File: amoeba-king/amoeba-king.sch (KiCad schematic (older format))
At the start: 6 parts, among them J1 Conn_01x05_Male, J2 Conn_01x05_Male, J3 Conn_01x04_Male, J4 Conn_01x05_Male, J5 Conn_01x01_Male, J6 Conn_01x01_Male

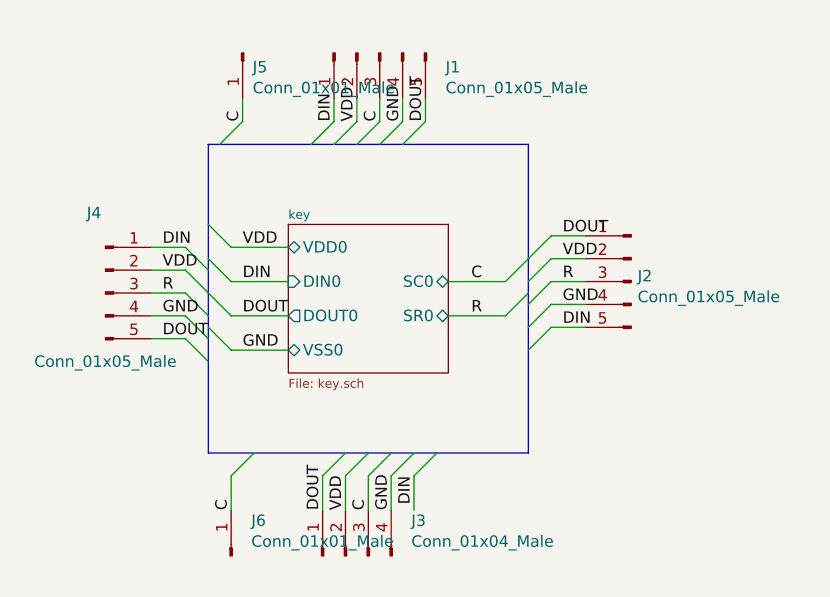
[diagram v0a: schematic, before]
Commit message: Getting pretty close to v1.1 improved Pads
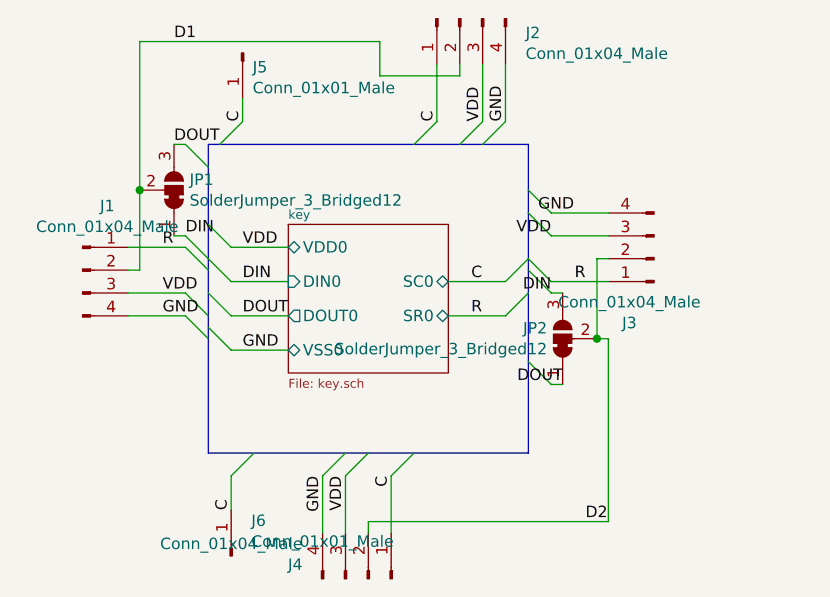
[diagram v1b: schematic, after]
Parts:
- removed J1, J2, J4: Conn_01x05_Male, amoeba-modules:Header_1x05_P1.27mm, symbol Connector:Conn_01x05_Male
- added J1, J4: Conn_01x04_Male, amoeba-modules:Header_1x04_P1.27mmL, symbol Connector:Conn_01x04_Male
- added J2: Conn_01x04_Male, amoeba-modules:Header_1x04_P1.27mm, symbol Connector:Conn_01x04_Male
- added JP1, JP2: SolderJumper_3_Bridged12, amoeba-modules:SolderJumper-3_P1.3mm_Open_RoundedPad1.0x1.5mm, symbol Jumper:SolderJumper_3_Bridged12
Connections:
- net C: now also J2.1 (Pin_1), J4.1 (Pin_1); no longer J3.3 (Pin_3)
- net DIN: now also JP1.1 (A), JP2.3 (B)
- net DOUT: now also JP1.3 (B), JP2.1 (A); no longer J3.1 (Pin_1)
- net GND: now also J1.4 (Pin_4), J2.4 (Pin_4), J4.4 (Pin_4)
- net R: now also J3.1 (Pin_1), J1.1 (Pin_1)
- net VDD: now also J3.3 (Pin_3), J1.3 (Pin_3), J2.3 (Pin_3), J4.3 (Pin_3); no longer J3.2 (Pin_2)
- new net D1: J1.2 (Pin_2), J2.2 (Pin_2), JP1.2 (C)
- new net D2: J3.2 (Pin_2), J4.2 (Pin_2), JP2.2 (C)
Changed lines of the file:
@@
 Text Label 4800 3500 0    50   ~ 0
 GND
-$Comp
-L Connector:Conn_01x05_Male J2
-U 1 1 5ED00D97
-P 6500 3200
-F 0 "J2" H 6472 3224 50  0000 R CNN
-F 1 "Conn_01x05_Male" H 6472 3133 50  0000 R CNN
-F 2 "amoeba-modules:Header_1x05_P1.27mm" H 6500 3200 50  0001 C CNN
-F 3 "~" H 6500 3200 50  0001 C CNN
-	1    6500 3200
-	-1   0    0    -1
-$EndComp
-$Comp
-L Connector:Conn_01x05_Male J4
-U 1 1 5ED02613
-P 4200 3250
-F 0 "J4" H 4150 3600 50  0000 C CNN
-F 1 "Conn_01x05_Male" H 4200 2950 50  0000 C CNN
-F 2 "amoeba-modules:Header_1x05_P1.27mm" H 4200 3250 50  0001 C CNN
-F 3 "~" H 4200 3250 50  0001 C CNN
-	1    4200 3250
-	1    0    0    -1
-$EndComp
-$Comp
-L Connector:Conn_01x05_Male J1
-U 1 1 5ED03164
-P 5400 2200
-F 0 "J1" V 5462 1912 50  0000 R CNN
-F 1 "Conn_01x05_Male" V 5553 1912 50  0000 R CNN
-F 2 "amoeba-modules:Header_1x05_P1.27mm" H 5400 2200 50  0001 C CNN
-F 3 "~" H 5400 2200 50  0001 C CNN
-	1    5400 2200
-	0    -1   1    0
-$EndComp
-Entry Wire Line
-	6050 3100 6150 3000
-Entry Wire Line
-	6050 3200 6150 3100
-Entry Wire Line
-	6050 3300 6150 3200
-Entry Wire Line
-	6050 3400 6150 3300
-Entry Wire Line
-	4550 3150 4650 3250
 Entry Wire Line
 	4550 3250 4650 3350
 Entry Wire Line
+	4550 3050 4650 3150
+Entry Wire Line
 	4550 3350 4650 3450
 Entry Wire Line
-	4550 3450 4650 3550
-Entry Wire Line
-	4550 3050 4650 3150
-Entry Wire Line
-	6050 3500 6150 3400
-Entry Wire Line
-	5100 2600 5200 2500
-Entry Wire Line
-	5200 2600 5300 2500
-Entry Wire Line
-	5300 2600 5400 2500
-Entry Wire Line
-	5400 2600 5500 2500
-Entry Wire Line
-	5500 2600 5600 2500
-Entry Wire Line
-	5150 4050 5250 3950
-Entry Wire Line
-	5250 4050 5350 3950
-Entry Wire Line
-	5350 4050 5450 3950
-Entry Wire Line
-	5450 4050 5550 3950
-Entry Wire Line
-	5550 4050 5650 3950
-Wire Wire Line
-	4400 3450 4550 3450
-Wire Wire Line
-	4550 3350 4400 3350
-Wire Wire Line
-	4550 3250 4400 3250
-Wire Wire Line
-	4550 3150 4400 3150
-Wire Wire Line
-	4550 3050 4400 3050
-Wire Wire Line
-	5200 2500 5200 2400
-Wire Wire Line
-	5300 2500 5300 2400
-Wire Wire Line
-	5400 2500 5400 2400
-Wire Wire Line
-	5500 2500 5500 2400
-Wire Wire Line
-	5600 2500 5600 2400
-Wire Wire Line
-	6150 3000 6300 3000
-Wire Wire Line
-	6150 3100 6300 3100
-Wire Wire Line
-	6150 3200 6300 3200
-Wire Wire Line
-	6150 3300 6300 3300
-Wire Wire Line
-	6150 3400 6300 3400
-Wire Wire Line
-	5550 4200 5550 4050
-Wire Wire Line
-	5450 4200 5450 4050
-Wire Wire Line
-	5350 4050 5350 4200
-Wire Wire Line
-	5250 4200 5250 4050
-Wire Wire Line
-	5150 4200 5150 4050
-Text Label 6200 3400 0    50   ~ 0
+	4550 2600 4650 2700
+Text Label 4450 3050 0    50   ~ 0
+R
+Text Label 4550 3000 0    50   ~ 0
 DIN
-Text Label 5200 2500 1    50   ~ 0
-DIN
-Text Label 5550 4050 3    50   ~ 0
-DIN
+Text Label 4500 2600 0    50   ~ 0
+DOUT
+Text Label 4450 3350 0    50   ~ 0
+GND
 Text Label 4450 3250 0    50   ~ 0
-R
-Text Label 6200 3200 0    50   ~ 0
-R
-Text Label 6200 3300 0    50   ~ 0
-GND
-Text Label 5500 2500 1    50   ~ 0
-GND
-Text Label 6200 3100 0    50   ~ 0
-VDD
-Text Label 5300 2500 1    50   ~ 0
-VDD
-Text Label 5600 2500 1    50   ~ 0
-DOUT
-Text Label 6200 3000 0    50   ~ 0
-DOUT
-Text Label 5150 4200 1    50   ~ 0
-DOUT
-Text Label 5350 4200 1    50   ~ 0
-C
-Text Label 5400 2500 1    50   ~ 0
-C
-Text Label 4450 3050 0    50   ~ 0
-DIN
-Text Label 4450 3450 0    50   ~ 0
-DOUT
-Text Label 5450 4200 1    50   ~ 0
-GND
-Text Label 5250 4200 1    50   ~ 0
-VDD
-Text Label 4450 3350 0    50   ~ 0
-GND
-Text Label 4450 3150 0    50   ~ 0
-VDD
-$Comp
-L Connector:Conn_01x04_Male J3
-U 1 1 5EC2A986
-P 5250 4400
-F 0 "J3" V 5404 4112 50  0000 R CNN
-F 1 "Conn_01x04_Male" V 5313 4112 50  0000 R CNN
-F 2 "amoeba-modules:Header_1x04_P1.27mm" H 5250 4400 50  0001 C CNN
-F 3 "~" H 5250 4400 50  0001 C CNN
-	1    5250 4400
-	0    -1   -1   0
-$EndComp
+VDD
 $Comp
 L Connector:Conn_01x01_Male J5
@@
 Text Label 4750 4200 1    50   ~ 0
 C
+$Comp
+L Jumper:SolderJumper_3_Bridged12 JP1
+U 1 1 5ECEDDD1
+P 4500 2800
+F 0 "JP1" V 4546 2868 50  0000 L CNN
+F 1 "SolderJumper_3_Bridged12" V 4455 2868 50  0000 L CNN
+F 2 "amoeba-modules:SolderJumper-3_P1.3mm_Open_RoundedPad1.0x1.5mm" H 4500 2800 50  0001 C CNN
+F 3 "~" H 4500 2800 50  0001 C CNN
+	1    4500 2800
+	0    1    -1   0
+$EndComp
+$Comp
+L Connector:Conn_01x04_Male J1
+U 1 1 5ECF294A
+P 4100 3150
+F 0 "J1" H 4208 3431 50  0000 C CNN
+F 1 "Conn_01x04_Male" H 4208 3340 50  0000 C CNN
+F 2 "amoeba-modules:Header_1x04_P1.27mmL" H 4100 3150 50  0001 C CNN
+F 3 "~" H 4100 3150 50  0001 C CNN
+	1    4100 3150
+	1    0    0    -1
+$EndComp
+Wire Wire Line
+	4300 3350 4550 3350
+Entry Wire Line
+	5750 2600 5850 2500
+Text Label 5850 2500 1    50   ~ 0
+VDD
+$Comp
+L Connector:Conn_01x04_Male J2
+U 1 1 5ED091AF
+P 5750 2050
+F 0 "J2" V 5812 1762 50  0000 R CNN
+F 1 "Conn_01x04_Male" V 5903 1762 50  0000 R CNN
+F 2 "amoeba-modules:Header_1x04_P1.27mm" H 5750 2050 50  0001 C CNN
+F 3 "~" H 5750 2050 50  0001 C CNN
+	1    5750 2050
+	0    -1   1    0
+$EndComp
+Text Label 5650 2500 1    50   ~ 0
+C
+Text Label 5950 2500 1    50   ~ 0
+GND
+Entry Wire Line
+	5850 2600 5950 2500
+Entry Wire Line
+	5550 2600 5650 2500
+Entry Wire Line
+	6150 3000 6050 2900
+Entry Wire Line
+	6150 3200 6050 3100
+Entry Wire Line
+	6150 2900 6050 2800
+Entry Wire Line
+	6150 3650 6050 3550
+Entry Wire Line
+	6150 3250 6050 3150
+Text Label 6300 3200 2    50   ~ 0
+R
+Text Label 6150 3250 2    50   ~ 0
+DIN
+Text Label 6200 3650 2    50   ~ 0
+DOUT
+Text Label 6250 2900 2    50   ~ 0
+GND
+Text Label 6150 3000 2    50   ~ 0
+VDD
+$Comp
+L Connector:Conn_01x04_Male J3
+U 1 1 5ED2E622
+P 6600 3100
+F 0 "J3" H 6708 3381 50  0000 C CNN
+F 1 "Conn_01x04_Male" H 6708 3290 50  0000 C CNN
+F 2 "amoeba-modules:Header_1x04_P1.27mm" H 6600 3100 50  0001 C CNN
+F 3 "~" H 6600 3100 50  0001 C CNN
+	1    6600 3100
+	-1   0    0    1
+$EndComp
+Wire Wire Line
+	6400 2900 6150 2900
+Entry Wire Line
+	4550 3000 4650 3100
+Wire Wire Line
+	4500 2600 4550 2600
+Wire Wire Line
+	4550 3000 4500 3000
+Wire Wire Line
+	6350 3450 6400 3450
+Wire Wire Line
+	6200 3250 6150 3250
+Wire Wire Line
+	6200 3650 6150 3650
+$Comp
+L Jumper:SolderJumper_3_Bridged12 JP2
+U 1 1 5ED2E618
+P 6200 3450
+F 0 "JP2" V 6246 3518 50  0000 L CNN
+F 1 "SolderJumper_3_Bridged12" V 6155 3518 50  0000 L CNN
+F 2 "amoeba-modules:SolderJumper-3_P1.3mm_Open_RoundedPad1.0x1.5mm" H 6200 3450 50  0001 C CNN
+F 3 "~" H 6200 3450 50  0001 C CNN
+	1    6200 3450
+	0    -1   -1   0
+$EndComp
+Wire Wire Line
+	5950 2250 5950 2500
+Entry Wire Line
+	5350 3950 5250 4050
+Text Label 5250 4050 3    50   ~ 0
+VDD
+$Comp
+L Connector:Conn_01x04_Male J4
+U 1 1 5ED66F35
+P 5350 4500
+F 0 "J4" V 5412 4212 50  0000 R CNN
+F 1 "Conn_01x04_Male" V 5503 4212 50  0000 R CNN
+F 2 "amoeba-modules:Header_1x04_P1.27mmL" H 5350 4500 50  0001 C CNN
+F 3 "~" H 5350 4500 50  0001 C CNN
+	1    5350 4500
+	0    1    -1   0
+$EndComp
+Text Label 5450 4050 3    50   ~ 0
+C
+Text Label 5150 4050 3    50   ~ 0
+GND
+Entry Wire Line
+	5250 3950 5150 4050
+Entry Wire Line
+	5550 3950 5450 4050
+Wire Wire Line
+	5150 4300 5150 4050
+Wire Wire Line
+	6400 3450 6400 4250
+Wire Wire Line
+	5400 2300 5400 2150
+Wire Wire Line
+	5400 2150 4350 2150
+Wire Wire Line
+	4350 2150 4350 2800
+Wire Wire Line
+	5450 4300 5450 4050
+Wire Wire Line
+	5650 2500 5650 2250
+Text Label 4500 2150 0    50   ~ 0
+D1
+Text Label 6300 4250 0    50   ~ 0
+D2
+Wire Wire Line
+	6150 3200 6400 3200
+Wire Wire Line
+	4550 3050 4300 3050
+Wire Wire Line
+	5850 2500 5850 2250
+Wire Wire Line
+	5750 2250 5750 2300
+Wire Wire Line
+	5750 2300 5400 2300
+Wire Wire Line
+	4300 3150 4350 3150
+Wire Wire Line
+	4350 3150 4350 2800
+Connection ~ 4350 2800
+Wire Wire Line
+	4550 3250 4300 3250
+Wire Wire Line
+	6150 3000 6400 3000
+Wire Wire Line
+	6400 3100 6350 3100
+Wire Wire Line
+	6350 3100 6350 3450
+Connection ~ 6350 3450
+Wire Wire Line
+	5250 4300 5250 4050
+Wire Wire Line
+	5350 4300 5350 4250
+Wire Wire Line
+	5350 4250 6400 4250
+Wire Bus Line
+	4650 3950 6050 3950
+Wire Bus Line
+	4650 2600 6050 2600
 Wire Bus Line
 	6050 2600 6050 3950
 Wire Bus Line
-	4650 2600 6050 2600
-Wire Bus Line
-	4650 3950 6050 3950
-Wire Bus Line
 	4650 2600 4650 3950
